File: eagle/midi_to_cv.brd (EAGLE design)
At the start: 100 x 80 mm, 46 parts, among them IC2 4504N, IC3 4099N, U1 ATMEGA328P_PDIP

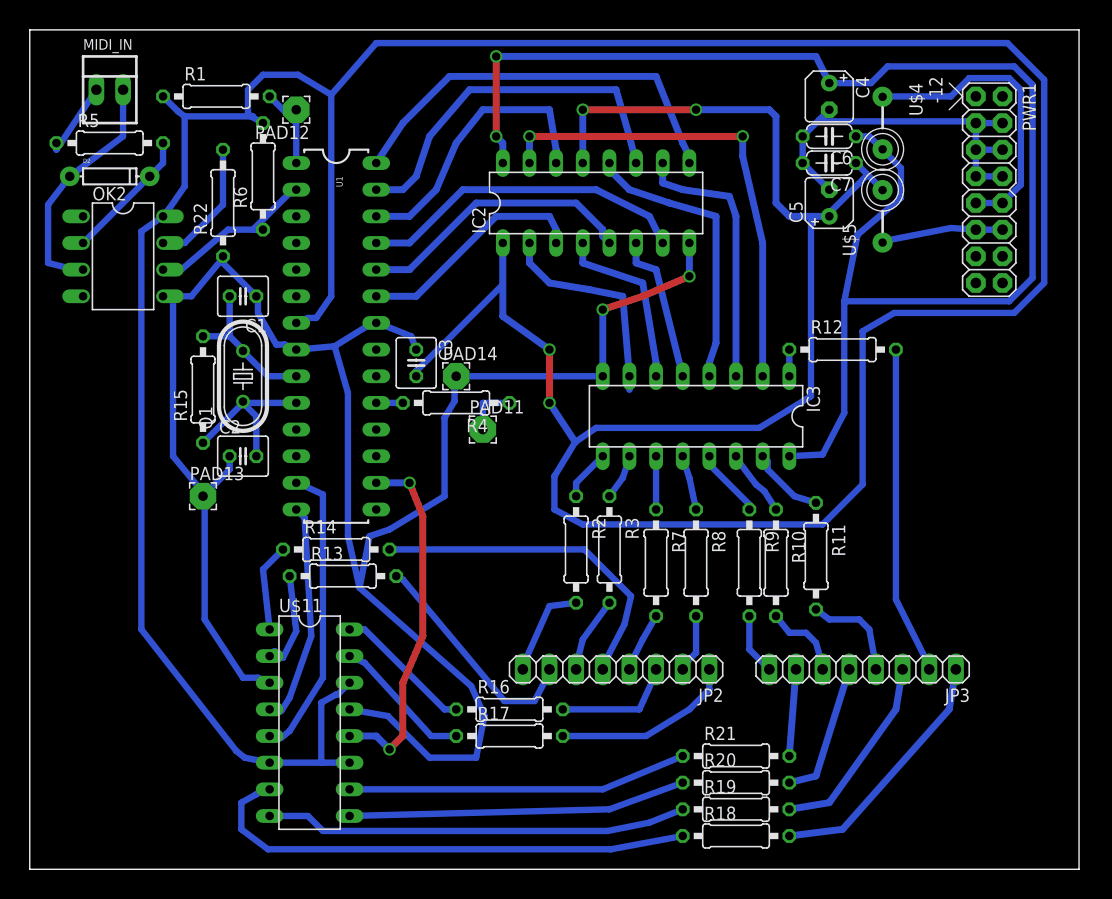
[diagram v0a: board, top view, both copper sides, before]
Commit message: cutout
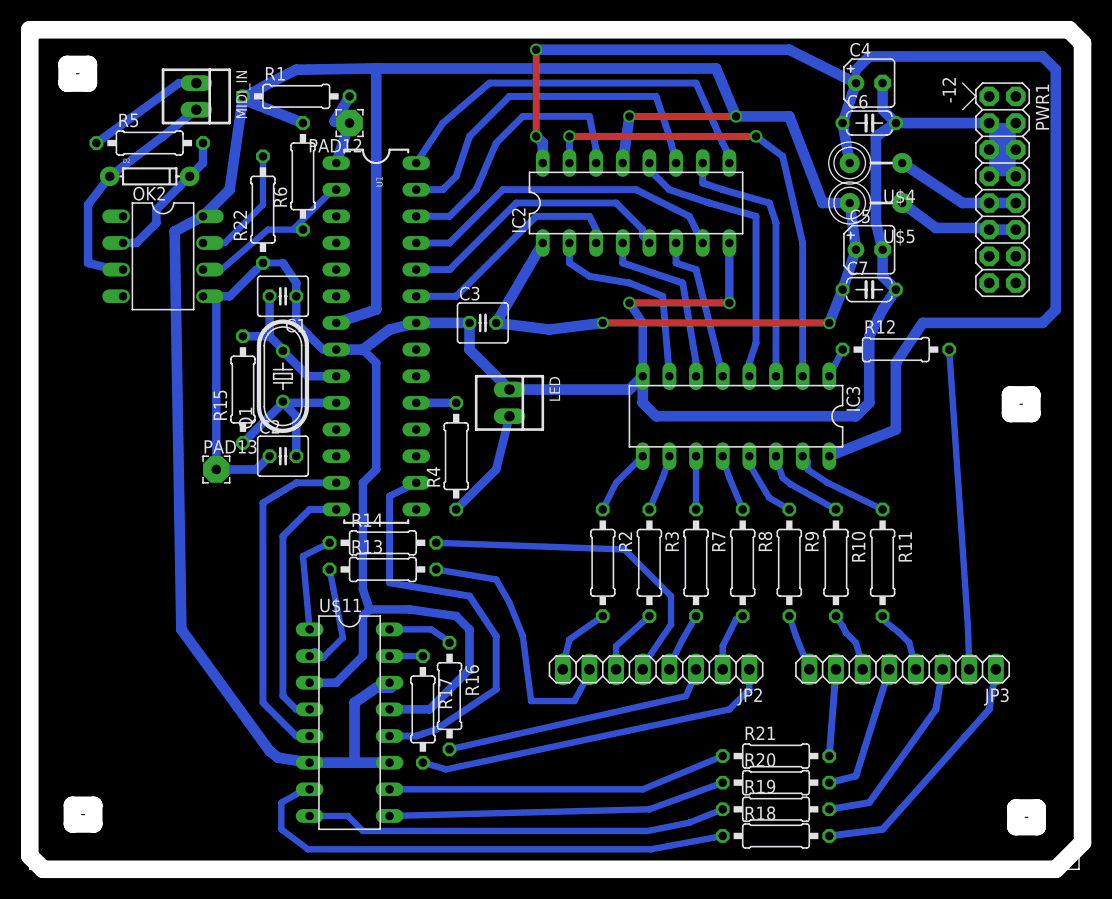
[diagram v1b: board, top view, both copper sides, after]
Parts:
- removed PAD11, PAD14: gate LED, wirepad:2,54/0,9
- added LED: 22-23-2021, con-molex:22-23-2021
- moved C7 12.7 mm to (80.0, 55.2), turned to 0 degrees
- moved R17 8.64 mm to (37.5, 15.2), turned to 270 degrees
- moved MIDI_IN 8.28 mm to (15.9, 73.7), turned to 270 degrees
- moved R1 7.62 mm to (25.4, 73.7)
- moved C3 7.41 mm to (43.2, 52.1), turned to 0 degrees
- moved R11 6.38 mm to (81.3, 29.2)
- moved C5 5.85 mm to (80.0, 59.1), turned to 0 degrees
- moved R16 5.85 mm to (40.0, 16.5), turned to 270 degrees
- moved R10 5.71 mm to (76.8, 29.2)
- moved PAD12 5.24 mm to (30.5, 71.1)
- moved R4 5.08 mm to (40.6, 39.4), turned to 90 degrees
- moved R12 5.08 mm to (82.5, 49.5)
- moved R14 4.49 mm to (33.7, 31.1)
- moved R8 4.44 mm to (67.9, 29.2)
- moved C4 4.02 mm to (80.0, 74.9), turned to 0 degrees
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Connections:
- removed net N$26: C4.-, C5.-, C6.2, C7.2, PWR1.3, PWR1.4, PWR1.5, PWR1.6, PWR1.7, PWR1.8
- net GND: now also C4.-, C5.-, C6.2, C7.2, LED.1, PWR1.3, PWR1.4, PWR1.5, PWR1.6, PWR1.7, PWR1.8; no longer PAD14.1
- net N$11: now also LED.2; no longer PAD11.1
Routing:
- net +5V: track 420.7 -> 258.0 mm
- net N$26: track 37.5 -> 0.00 mm
- net GND: track 195.6 -> 226.4 mm
- net N$29: track 17.4 -> 34.5 mm
- net N$2: track 28.5 -> 12.0 mm
- net +12V: track 140.3 -> 125.4 mm
- net N$28: track 11.5 -> 25.8 mm
- net N$55: track 13.4 -> 3.33 mm
- net N$54: track 13.3 -> 6.42 mm
- net N$15: track 34.1 -> 39.9 mm, vias 2 -> 0
- net N$11: track 5.08 -> 10.6 mm
- net N$14: track 28.4 -> 32.3 mm
- net N$19: track 7.50 -> 11.4 mm
- net N$22: track 22.0 -> 25.5 mm
- net N$16: track 9.66 -> 6.32 mm
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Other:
- board size 100 x 80 mm -> 100.3 x 80 mm
